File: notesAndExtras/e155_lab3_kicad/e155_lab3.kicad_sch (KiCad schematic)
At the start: 16 parts, among them SW1 SW_DIP_x08

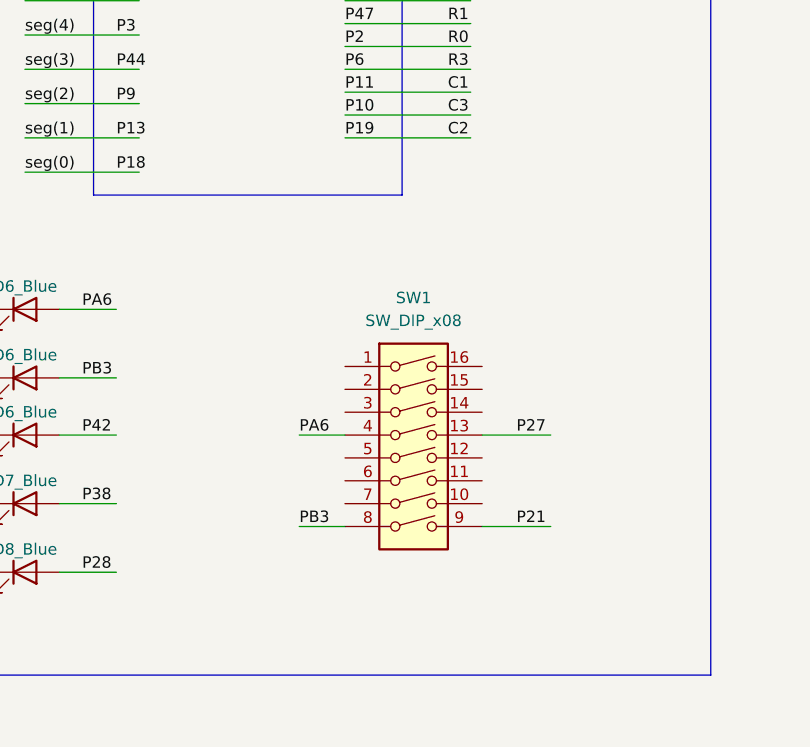
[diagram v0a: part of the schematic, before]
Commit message: Update Schematic
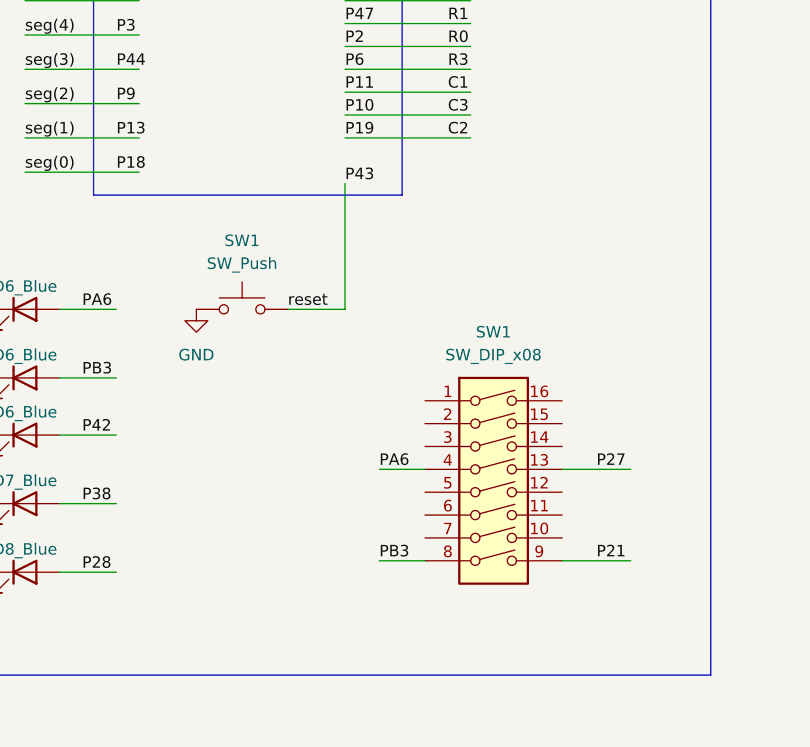
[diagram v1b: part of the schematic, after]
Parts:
- added SW1: SW_Push, symbol Switch:SW_Push
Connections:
- net GND: now also SW1.1
- new net P43: SW1.2
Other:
- moved on the sheet: SW1
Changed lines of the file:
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@@
     (stroke (width 0) (type default))
   )
-  (wire (pts (xy 71.12 144.78) (xy 76.2 144.78))
+  (wire (pts (xy 80.01 148.59) (xy 85.09 148.59))
     (stroke (width 0) (type default))
   )
@@
     (stroke (width 0) (type default))
   )
+  (wire (pts (xy 76.2 106.68) (xy 76.2 120.65))
+    (stroke (width 0) (type default))
+  )
   (wire (pts (xy 157.48 132.08) (xy 165.1 132.08))
     (stroke (width 0) (type default))
@@
     (stroke (width 0) (type default))
   )
-  (wire (pts (xy 71.12 134.62) (xy 76.2 134.62))
+  (wire (pts (xy 80.01 138.43) (xy 85.09 138.43))
     (stroke (width 0) (type default))
   )
@@
     (stroke (width 0) (type default))
   )
-  (wire (pts (xy 91.44 134.62) (xy 99.06 134.62))
+  (wire (pts (xy 100.33 138.43) (xy 107.95 138.43))
     (stroke (width 0) (type default))
   )
@@
     (stroke (width 0) (type default))
   )
-  (wire (pts (xy 91.44 144.78) (xy 99.06 144.78))
+  (wire (pts (xy 100.33 148.59) (xy 107.95 148.59))
     (stroke (width 0) (type default))
   )
@@
   )
   (wire (pts (xy 195.58 132.08) (xy 205.74 132.08))
+    (stroke (width 0) (type default))
+  )
+  (wire (pts (xy 69.85 120.65) (xy 76.2 120.65))
     (stroke (width 0) (type default))
   )
@@
     (effects (font (size 2 2)) (justify left bottom))
   )
+  (label "reset" (at 69.85 120.65 0) (fields_autoplaced)
+    (effects (font (size 1.27 1.27)) (justify left bottom))
+  )
   (label "R0" (at 182.88 97.79 0) (fields_autoplaced)
     (effects (font (size 1.27 1.27)) (justify left bottom))
@@
     (effects (font (size 1.27 1.27)) (justify left bottom))
   )
-  (label "PA6" (at 71.12 134.62 0) (fields_autoplaced)
+  (label "PA6" (at 80.01 138.43 0) (fields_autoplaced)
     (effects (font (size 1.27 1.27)) (justify left bottom))
   )
@@
     (effects (font (size 1.27 1.27)) (justify left bottom))
   )
-  (label "P27" (at 95.25 134.62 0) (fields_autoplaced)
+  (label "P27" (at 104.14 138.43 0) (fields_autoplaced)
     (effects (font (size 1.27 1.27)) (justify left bottom))
   )
@@
     (effects (font (size 1.27 1.27)) (justify left bottom))
   )
-  (label "PB3" (at 71.12 144.78 0) (fields_autoplaced)
+  (label "PB3" (at 80.01 148.59 0) (fields_autoplaced)
     (effects (font (size 1.27 1.27)) (justify left bottom))
   )
@@
     (effects (font (size 2 2)) (justify left bottom))
   )
+  (label "P43" (at 76.2 106.68 0) (fields_autoplaced)
+    (effects (font (size 1.27 1.27)) (justify left bottom))
+  )
   (label "Pin 8" (at 214.63 77.47 90) (fields_autoplaced)
     (effects (font (size 1.27 1.27)) (justify left bottom))
@@
     (effects (font (size 1.27 1.27)) (justify left bottom))
   )
-  (label "P21" (at 95.25 144.78 0) (fields_autoplaced)
+  (label "P21" (at 104.14 148.59 0) (fields_autoplaced)
     (effects (font (size 1.27 1.27)) (justify left bottom))
   )
@@
     )
   )
+  (symbol (lib_id "power:GND") (at 59.69 120.65 0) (unit 1)
+    (in_bom yes) (on_board yes) (dnp no) (fields_autoplaced)
+    (property "Reference" "#PWR04" (at 59.69 127 0)
+      (effects (font (size 1.27 1.27)) hide)
+    )
+    (property "Value" "GND" (at 59.69 125.73 0)
+      (effects (font (size 1.27 1.27)))
+    )
+    (property "Footprint" "" (at 59.69 120.65 0)
+      (effects (font (size 1.27 1.27)) hide)
+    )
+    (property "Datasheet" "" (at 59.69 120.65 0)
+      (effects (font (size 1.27 1.27)) hide)
+    )
+    (pin "1")
+    (instances
+      (project "e155_lab1_schematic"
+        (path "/b185a060-64b9-486b-bf7d-f6a41fb3eb98"
+          (reference "#PWR04") (unit 1)
+        )
+      )
+      (project "e155_lab3"
+        (path "/b3f22ff6-ab3f-4a03-b10e-5d7cba55f4ec"
+          (reference "#PWR04") (unit 1)
+        )
+      )
+    )
+  )
   (symbol (lib_id "Device:R_US") (at 139.7 55.88 90) (unit 1)
     (in_bom yes) (on_board yes) (dnp no)
@@
         (path "/d7354254-033c-4a0e-abd9-0ea0bac08356"
           (reference "Rb1") (unit 1)
+        )
+      )
+    )
+  )
+  (symbol (lib_id "Switch:SW_Push") (at 64.77 120.65 0) (unit 1)
+    (in_bom yes) (on_board yes) (dnp no)
+    (property "Reference" "SW1" (at 64.77 113.03 0)
+      (effects (font (size 1.27 1.27)))
+    )
+    (property "Value" "SW_Push" (at 64.77 115.57 0)
+      (effects (font (size 1.27 1.27)))
+    )
+    (property "Footprint" "" (at 64.77 115.57 0)
+      (effects (font (size 1.27 1.27)) hide)
+    )
+    (property "Datasheet" "~" (at 64.77 115.57 0)
+      (effects (font (size 1.27 1.27)) hide)
+    )
+    (pin "1")
+    (pin "2")
+    (instances
+      (project "e155_lab1_schematic"
+        (path "/b185a060-64b9-486b-bf7d-f6a41fb3eb98"
+          (reference "SW1") (unit 1)
+        )
+      )
+      (project "e155_lab3"
+        (path "/b3f22ff6-ab3f-4a03-b10e-5d7cba55f4ec"
+          (reference "SW2") (unit 1)
         )
       )
@@
     )
   )
-  (symbol (lib_id "Switch:SW_DIP_x08") (at 83.82 137.16 0) (unit 1)
+  (symbol (lib_id "Switch:SW_DIP_x08") (at 92.71 140.97 0) (unit 1)
     (in_bom yes) (on_board yes) (dnp no) (fields_autoplaced)
-    (property "Reference" "SW1" (at 83.82 119.38 0)
-      (effects (font (size 1.27 1.27)))
-    )
-    (property "Value" "SW_DIP_x08" (at 83.82 121.92 0)
-      (effects (font (size 1.27 1.27)))
-    )
-    (property "Footprint" "" (at 83.82 137.16 0)
-      (effects (font (size 1.27 1.27)) hide)
-    )
-    (property "Datasheet" "~" (at 83.82 137.16 0)
-      (effects (font (size 1.27 1.27)) hide)
-    )
+    (property "Reference" "SW1" (at 92.71 123.19 0)
+      (effects (font (size 1.27 1.27)))
+    )
+    (property "Value" "SW_DIP_x08" (at 92.71 125.73 0)
+      (effects (font (size 1.27 1.27)))
+    )
+    (property "Footprint" "" (at 92.71 140.97 0)
+      (effects (font (size 1.27 1.27)) hide)
+    )
+    (property "Datasheet" "~" (at 92.71 140.97 0)
+      (effects (font (size 1.27 1.27)) hide)
+    )
